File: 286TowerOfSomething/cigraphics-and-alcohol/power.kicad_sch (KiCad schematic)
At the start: 1 part, among them U1 TVGA9000I-3

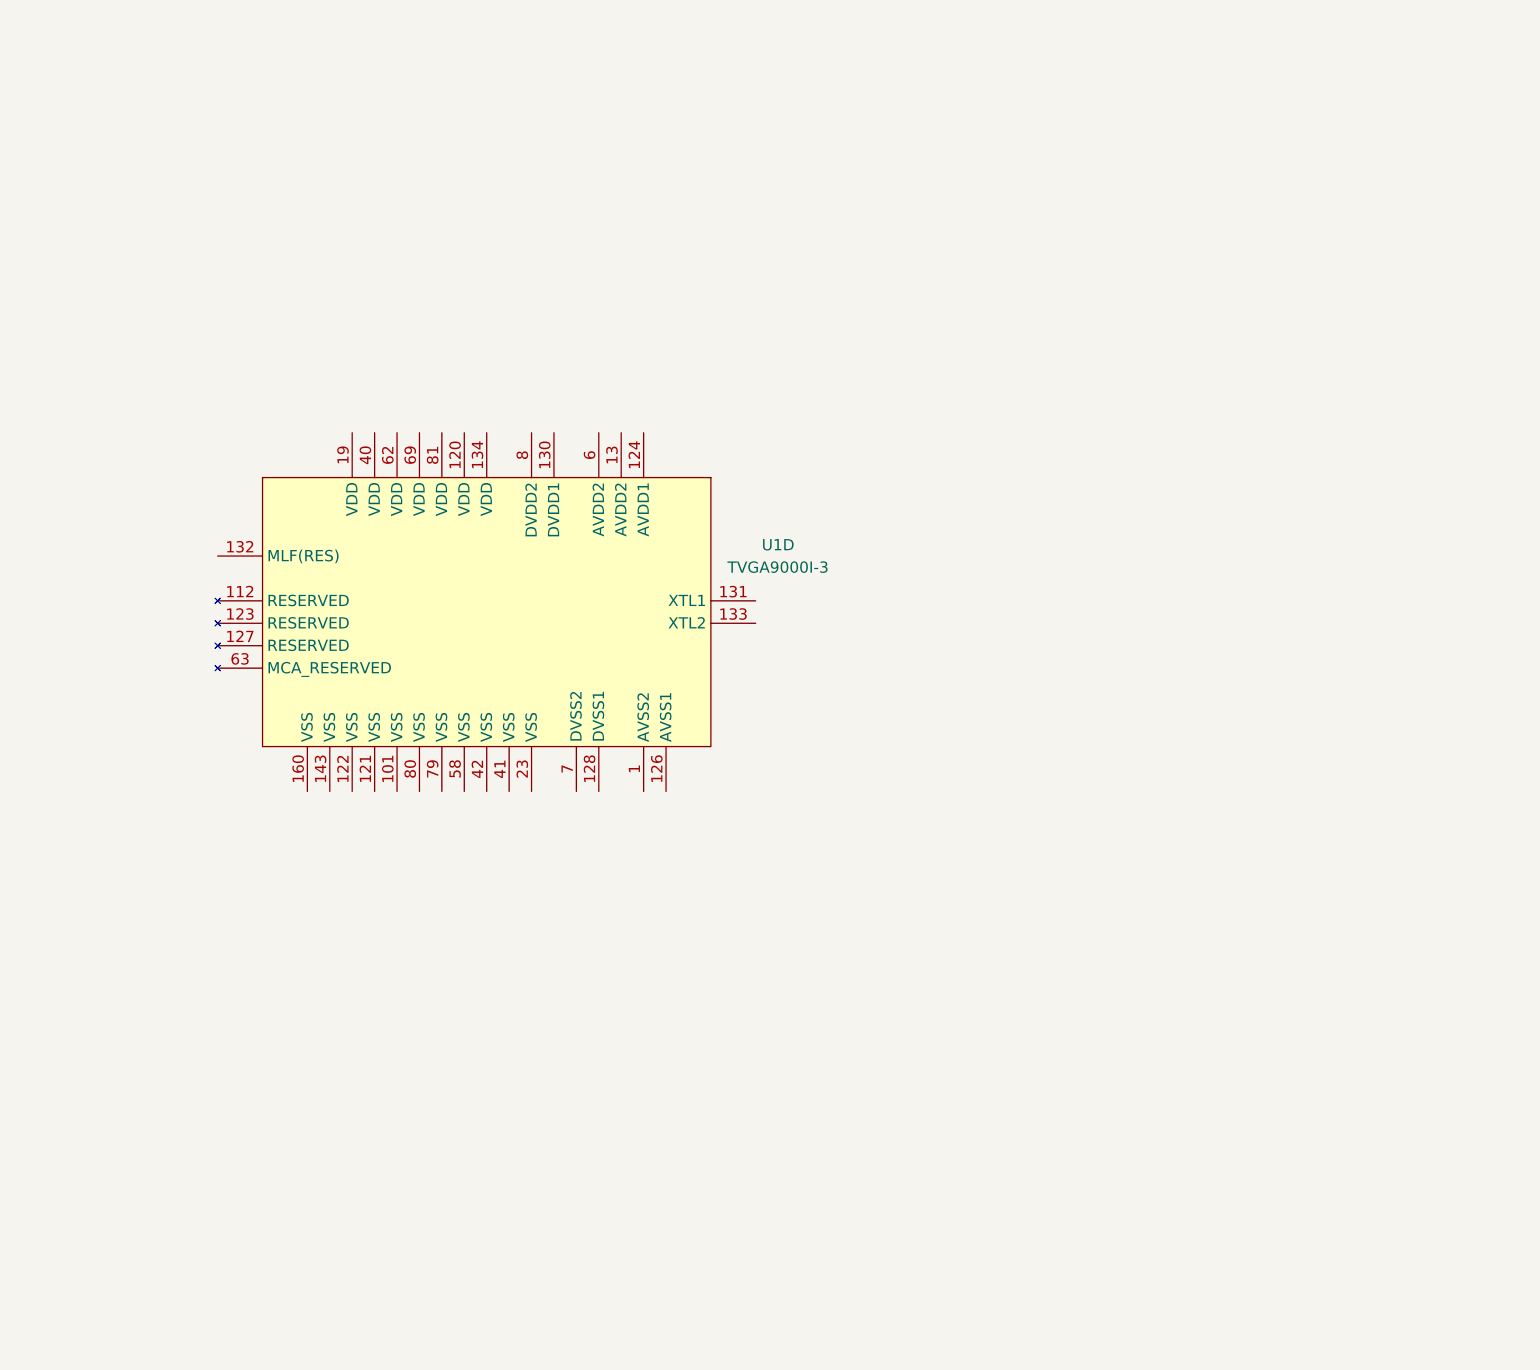
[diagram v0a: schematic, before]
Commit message: Almost finished schematic for cigraphics-and-alcohol
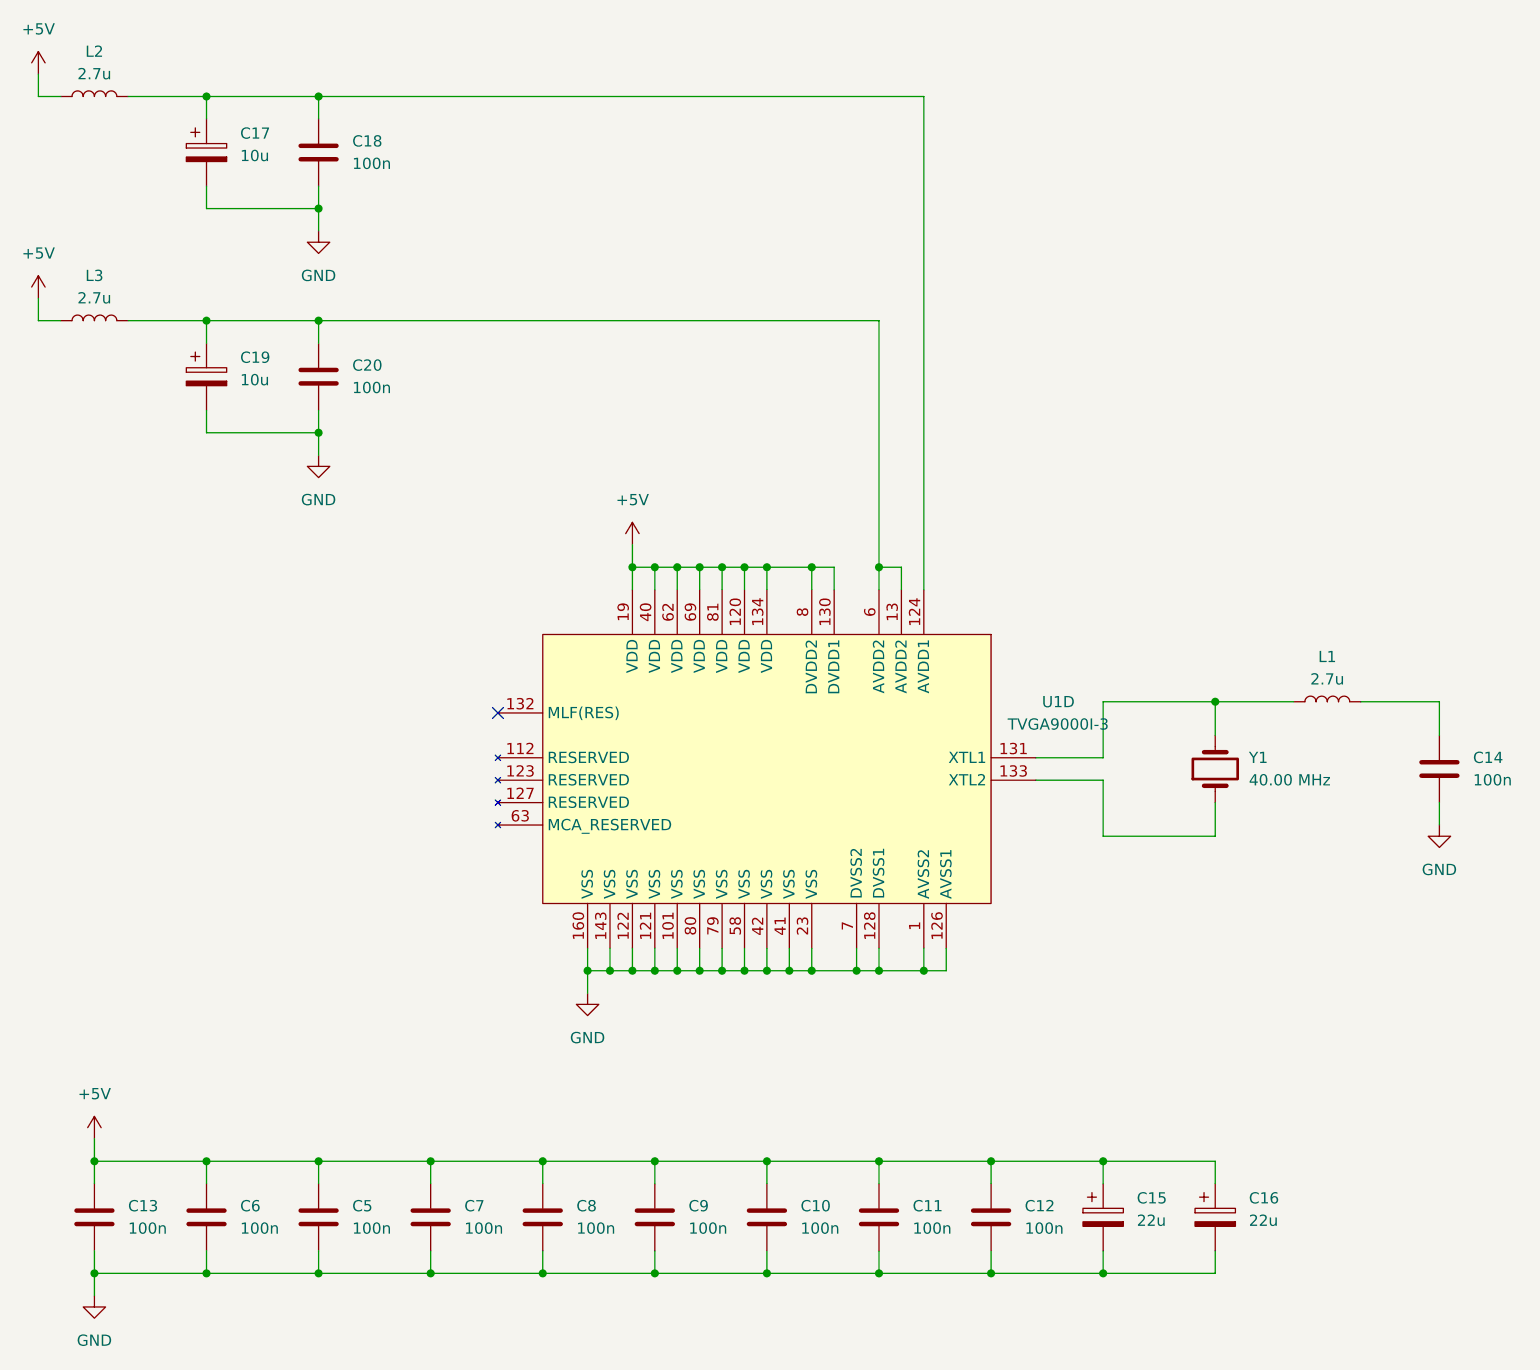
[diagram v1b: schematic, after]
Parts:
- added C10, C11, C12, C13, C14, C18, C20, C5, C6, C7, C8, C9: 100n, Capacitor_SMD:C_0603_1608Metric_Pad1.08x0.95mm_HandSolder, symbol Device:C
- added C15, C16: 22u, Capacitor_SMD:CP_Elec_5x5.3, symbol Device:C_Polarized
- added C17, C19: 10u, Capacitor_SMD:CP_Elec_5x5.3, symbol Device:C_Polarized
- added L1, L2, L3: 2.7u, Inductor_SMD:L_0603_1608Metric_Pad1.05x0.95mm_HandSolder, symbol Device:L
- added Y1: 40.00 MHz, symbol Device:Crystal
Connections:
- net GND: now reaches U1.1 (AVSS2)
- net GND: now also U1.101 (VSS), U1.121 (VSS), U1.122 (VSS), U1.126 (AVSS1), U1.128 (DVSS1), U1.143 (VSS), U1.160 (VSS), U1.23 (VSS), U1.41 (VSS), U1.42 (VSS), U1.58 (VSS), U1.7 (DVSS2), U1.79 (VSS), U1.80 (VSS), C10.2, C11.2, C12.2, C13.2, C14.2, C15.2, C16.2, C17.2, C18.2, C19.2, C20.2, C5.2, C6.2, C7.2, C8.2, C9.2
- net +5V: now reaches U1.120 (VDD)
- net +5V: now also U1.130 (DVDD1), U1.134 (VDD), U1.19 (VDD), U1.40 (VDD), U1.62 (VDD), U1.69 (VDD), U1.8 (DVDD2), U1.81 (VDD), C10.1, C11.1, C12.1, C13.1, C15.1, C16.1, C5.1, C6.1, C7.1, C8.1, C9.1, L2.1, L3.1
- net at U1.124 (AVDD1): now also C17.1, C18.1, L2.2
- net at U1.13 (AVDD2): now also U1.6 (AVDD2), C19.1, C20.1, L3.2
- net at U1.131 (XTL1): now also L1.1, Y1.2
- net at U1.133 (XTL2): now also Y1.1
- new net: C14.1, L1.2
- no-connect marks 0 -> 1
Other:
- moved on the sheet: U1D

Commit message: Adding bracket to graphics card
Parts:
- Y1: footprint (none) -> Crystal:Crystal_HC49-4H_Vertical
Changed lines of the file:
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@@
 			)
 		)
-		(property "Footprint" ""
+		(property "Footprint" "Crystal:Crystal_HC49-4H_Vertical"
 			(at 177.8 101.6 0)
 			(effects
